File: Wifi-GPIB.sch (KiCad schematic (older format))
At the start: 10 parts

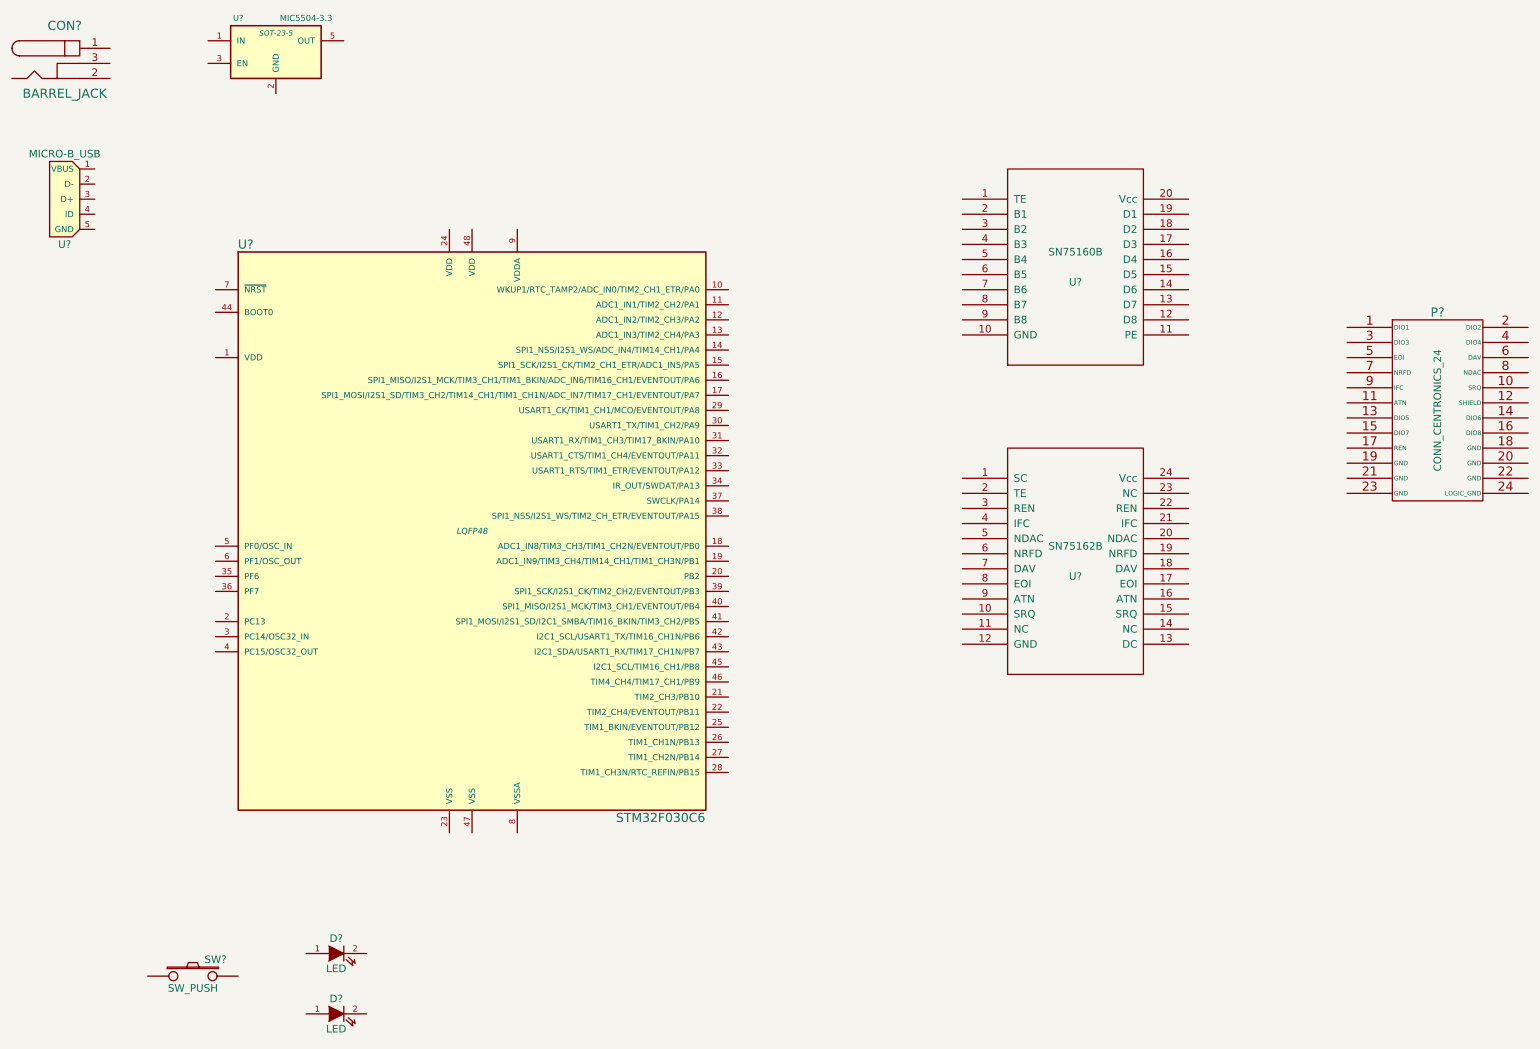
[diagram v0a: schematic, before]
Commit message: Add ESP to sch
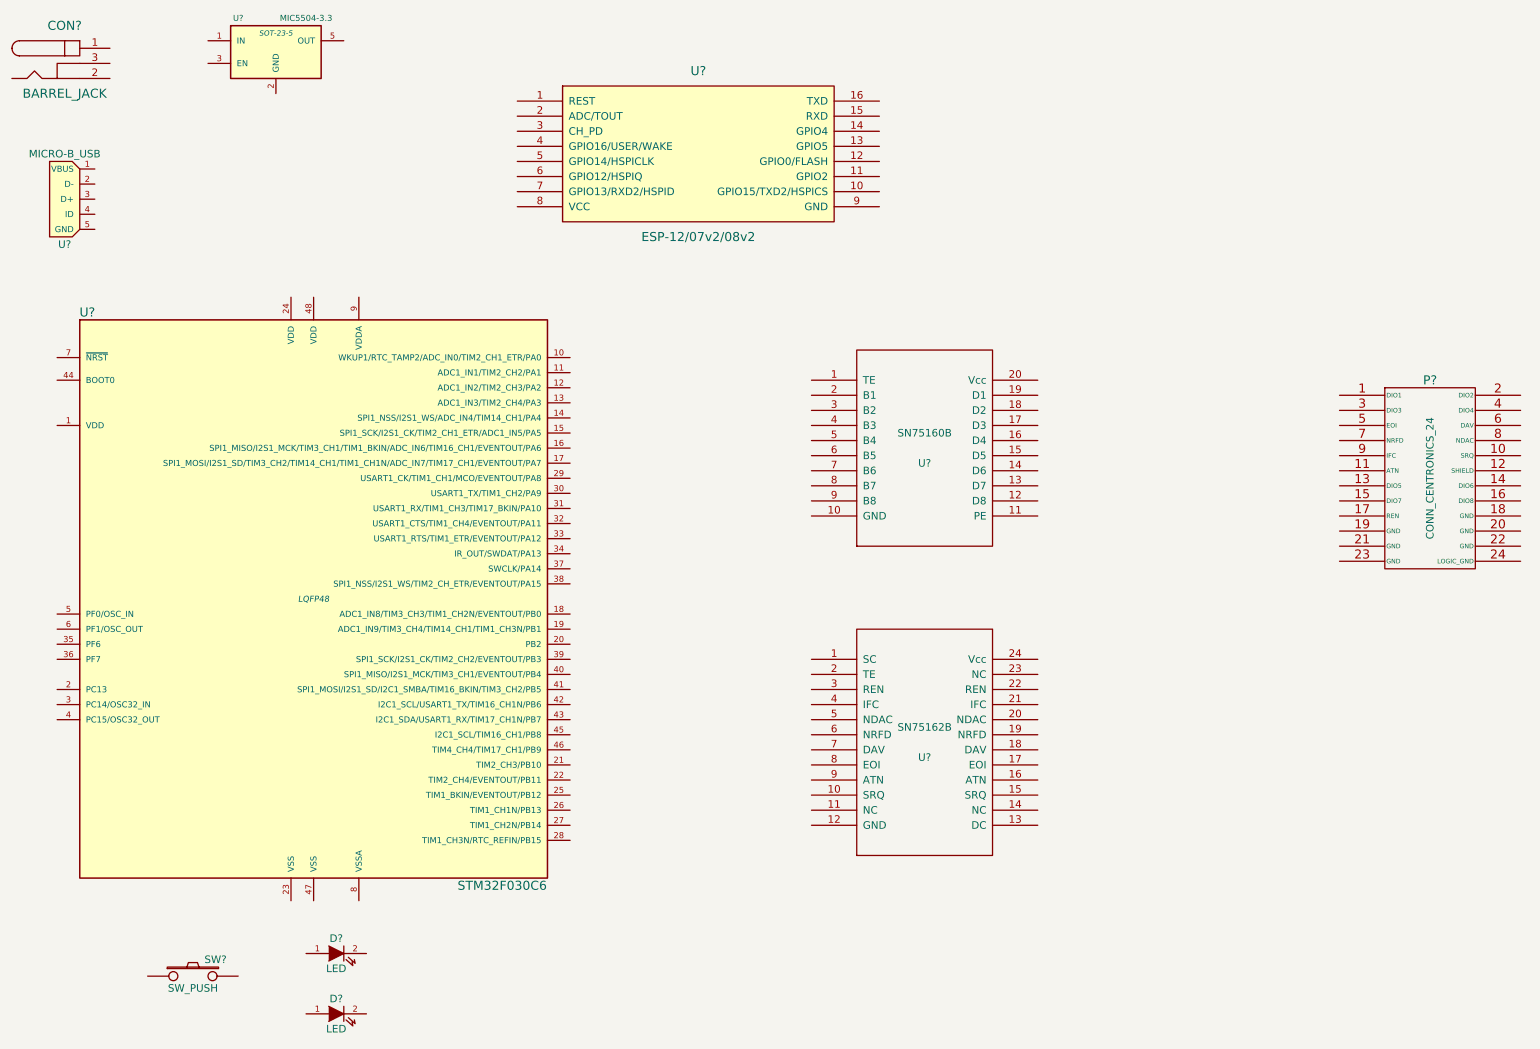
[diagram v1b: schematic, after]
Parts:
- added U?: ESP-12/07v2/08v2, symbol ESP-12/07v2/08v2
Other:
- moved on the sheet: P?, U?
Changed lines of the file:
@@
 LIBS:open-project
 LIBS:mic5504
+LIBS:esp8266
+LIBS:Wifi-GPIB-cache
 EELAYER 25 0
 EELAYER END
@@
 L STM32F030C6 U?
 U 1 1 5564BC8B
-P 3950 4100
-F 0 "U?" H 2450 6000 60  0000 C CNN
-F 1 "STM32F030C6" H 5200 2200 60  0000 C CNN
-F 2 "LQFP48" H 3950 4100 40  0000 C CIN
-F 3 "" H 3950 4100 60  0000 C CNN
-	1    3950 4100
+P 2900 4550
+F 0 "U?" H 1400 6450 60  0000 C CNN
+F 1 "STM32F030C6" H 4150 2650 60  0000 C CNN
+F 2 "LQFP48" H 2900 4550 40  0000 C CIN
+F 3 "" H 2900 4550 60  0000 C CNN
+	1    2900 4550
 	1    0    0    -1
 $EndComp
@@
 L SN75160B U?
 U 1 1 5564BDA6
-P 7950 2350
-F 0 "U?" H 7950 2250 50  0000 C CNN
-F 1 "SN75160B" H 7950 2450 50  0000 C CNN
-F 2 "MODULE" H 7950 2350 50  0001 C CNN
-F 3 "DOCUMENTATION" H 7950 2350 50  0001 C CNN
-	1    7950 2350
+P 6950 3550
+F 0 "U?" H 6950 3450 50  0000 C CNN
+F 1 "SN75160B" H 6950 3650 50  0000 C CNN
+F 2 "MODULE" H 6950 3550 50  0001 C CNN
+F 3 "DOCUMENTATION" H 6950 3550 50  0001 C CNN
+	1    6950 3550
 	1    0    0    -1
 $EndComp
@@
 L SN75162B U?
 U 1 1 5564BE4F
-P 7950 4300
-F 0 "U?" H 7950 4200 50  0000 C CNN
-F 1 "SN75162B" H 7950 4400 50  0000 C CNN
-F 2 "MODULE" H 7950 4300 50  0001 C CNN
-F 3 "DOCUMENTATION" H 7950 4300 50  0001 C CNN
-	1    7950 4300
+P 6950 5500
+F 0 "U?" H 6950 5400 50  0000 C CNN
+F 1 "SN75162B" H 6950 5600 50  0000 C CNN
+F 2 "MODULE" H 6950 5500 50  0001 C CNN
+F 3 "DOCUMENTATION" H 6950 5500 50  0001 C CNN
+	1    6950 5500
 	1    0    0    -1
 $EndComp
@@
 L CONN_CENTRONICS_24 P?
 U 1 1 5564D4E2
-P 10350 3300
-F 0 "P?" H 10350 3950 60  0000 C CNN
-F 1 "CONN_CENTRONICS_24" V 10350 3300 50  0000 C CNN
-F 2 "" H 10350 3300 60  0000 C CNN
-F 3 "" H 10350 3300 60  0000 C CNN
-	1    10350 3300
+P 10300 3750
+F 0 "P?" H 10300 4400 60  0000 C CNN
+F 1 "CONN_CENTRONICS_24" V 10300 3750 50  0000 C CNN
+F 2 "" H 10300 3750 60  0000 C CNN
+F 3 "" H 10300 3750 60  0000 C CNN
+	1    10300 3750
 	1    0    0    -1
 $EndComp
@@
 	1    0    0    -1
 $EndComp
+$Comp
+L ESP-12/07v2/08v2 U?
+U 1 1 5564D82B
+P 5450 1600
+F 0 "U?" H 5450 2150 60  0000 C CNN
+F 1 "ESP-12/07v2/08v2" H 5450 1050 60  0000 C CNN
+F 2 "" H 5450 1600 60  0000 C CNN
+F 3 "" H 5450 1600 60  0000 C CNN
+	1    5450 1600
+	1    0    0    -1
+$EndComp
